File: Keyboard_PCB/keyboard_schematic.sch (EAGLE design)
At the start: 262 parts, among them J1 1-2295018-2, M2 KEYSWITCH-RGBSMDLED-ALPSMX-1U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, M3 KEYSWITCH-RGBSMDLED-ALPSMX-1U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, M4 KEYSWITCH-RGBSMDLED-ALPSMX-1U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, M5 KEYSWITCH-RGBSMDLED-ALPSMX-1U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, M6 KEYSWITCH-RGBSMDLED-ALPSMX-1U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, Y2 CRYSTAL-GROUNDEDSMD-3.2X2.5

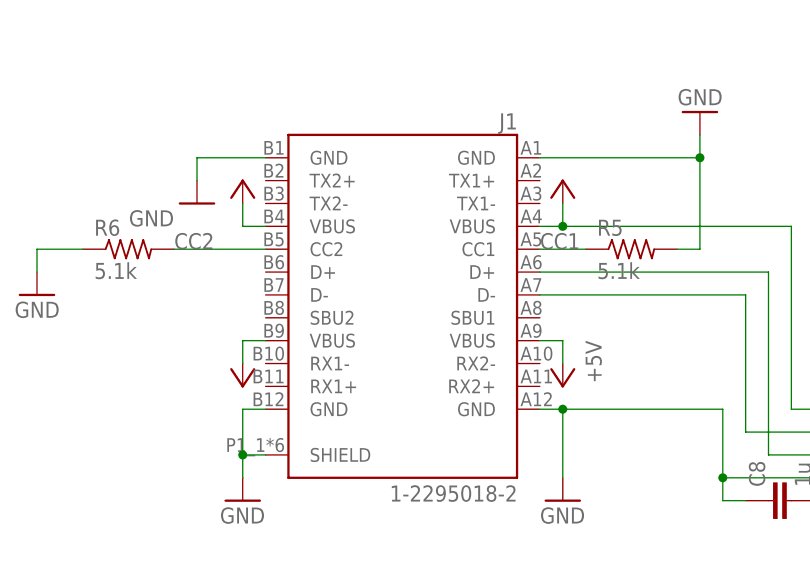
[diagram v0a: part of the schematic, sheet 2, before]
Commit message: Updated Board
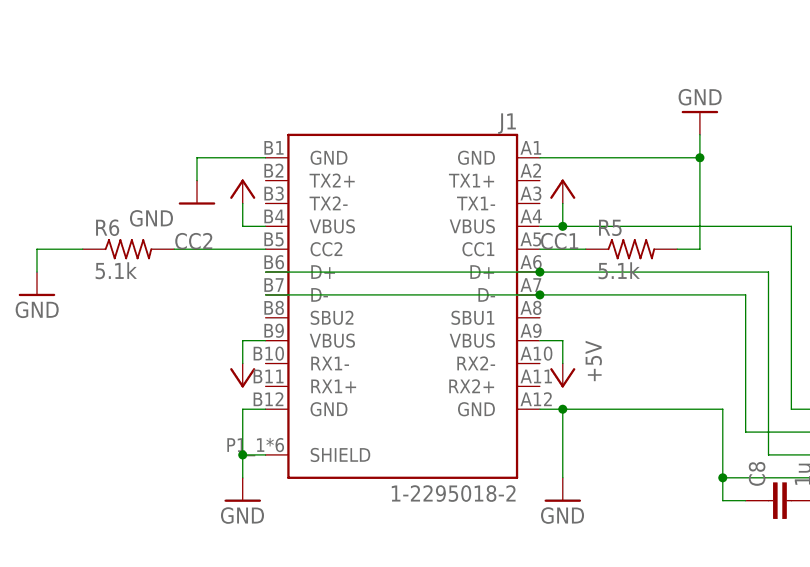
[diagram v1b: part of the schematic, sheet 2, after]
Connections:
- net D+USB: now also J1.D+@1
- net D-USB: now also J1.D-@1
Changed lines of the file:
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@@
 <sheets>
 <sheet>
+<description>Key connections</description>
 <plain>
 </plain>
@@
 </sheet>
 <sheet>
-<description>Main Board</description>
+<description>Controller Board</description>
 <plain>
 </plain>
@@
 <pinref part="J1" gate="G$1" pin="D+"/>
 <wire x1="-162.56" y1="71.12" x2="-137.16" y2="71.12" width="0.1524" layer="91"/>
+<pinref part="J1" gate="G$1" pin="D+@1"/>
+<wire x1="-193.04" y1="71.12" x2="-162.56" y2="71.12" width="0.1524" layer="91"/>
+<junction x="-162.56" y="71.12"/>
 </segment>
 </net>
@@
 <pinref part="J1" gate="G$1" pin="D-"/>
 <wire x1="-162.56" y1="68.58" x2="-139.7" y2="68.58" width="0.1524" layer="91"/>
+<pinref part="J1" gate="G$1" pin="D-@1"/>
+<wire x1="-162.56" y1="68.58" x2="-193.04" y2="68.58" width="0.1524" layer="91"/>
+<junction x="-162.56" y="68.58"/>
 </segment>
 </net>
